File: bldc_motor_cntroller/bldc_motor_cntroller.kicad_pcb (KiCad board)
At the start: 4 copper layers, 85.5 x 56 mm, 230 parts, among them J1 MR30PW-M 15A (30A), J10 Conn_01x05, J11 Conn_01x05, J2 MR30PW-M 15A (30A), J3 XT30, J4 USB_C_Receptacle_USB2.0, J5 Conn_01x03, J6 Conn_01x06, J7 Conn_01x02, J8 Conn_01x02, J9 Conn_01x04, Q1 IRF7480MTRPBF, Q10 IRF7480MTRPBF, Q11 IRF7480MTRPBF, Q12 IRF7480MTRPBF, Q13 CSD18540Q5B, Q14 CSD18540Q5B, Q2 IRF7480MTRPBF, Q3 IRF7480MTRPBF, Q4 IRF7480MTRPBF, Q5 IRF7480MTRPBF, Q6 IRF7480MTRPBF, Q7 IRF7480MTRPBF, Q8 IRF7480MTRPBF, Q9 IRF7480MTRPBF, SW1 B3U-1000P-B, U1 DRV8301DCAR, U2 DRV8301DCAR, U3 LM5109BSD, U4 SPX3819M5-L-3-3, U5 LP5907MFX-3.3, U6 STM32F405RGTx, U7 SN65HVD232, U8 USBLC6-2SC6, Y1 Crystal_GND3_Small

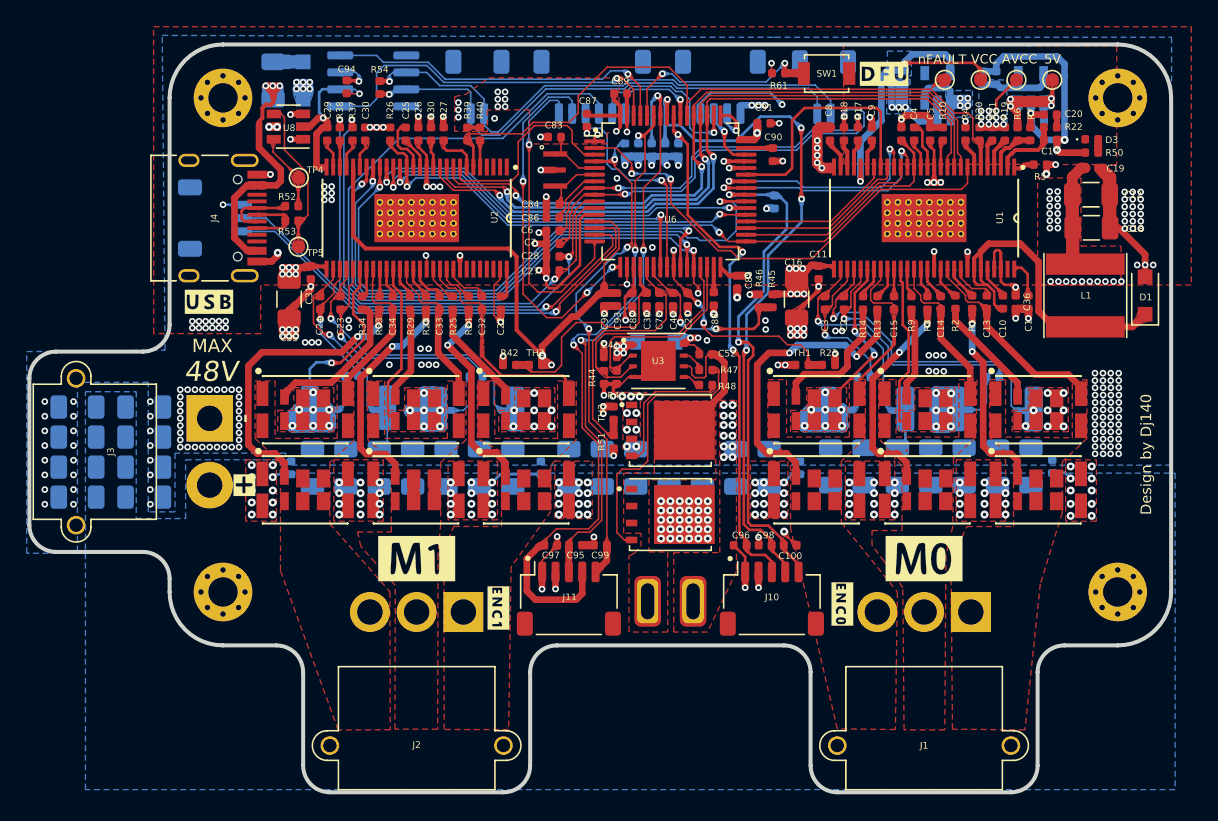
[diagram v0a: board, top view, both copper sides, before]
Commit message: Kicad 10
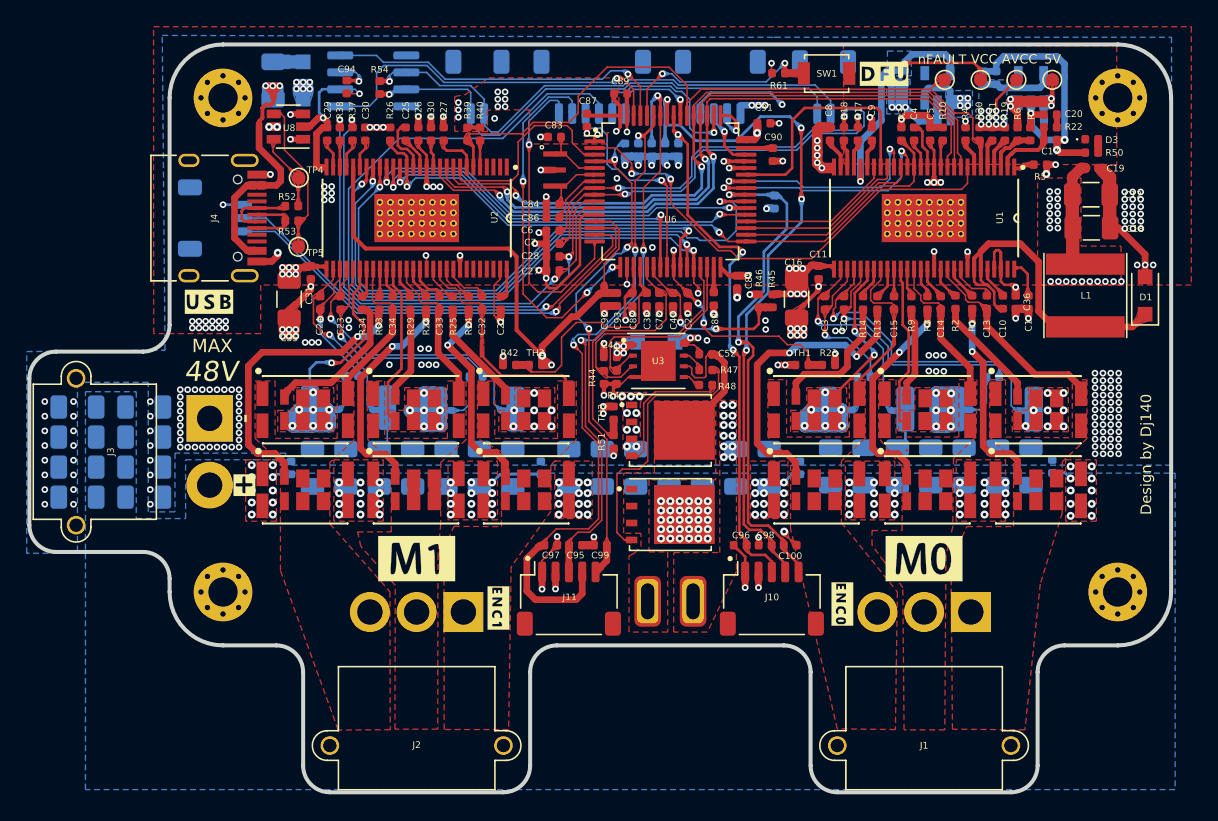
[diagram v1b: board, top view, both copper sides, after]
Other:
- net class Default removed
- net class HV removed
